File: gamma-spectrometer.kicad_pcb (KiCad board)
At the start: 2 copper layers, 123.5 x 49.5 mm, 79 parts, among them J1 *, J2 *, J3 20449-001E-03, J4 *, J5 20449-001E-03, J6 *, Q1 2N7002, Q2 2N7002, Q3 MMBT5088LT1G, Q4 MMBT5088LT1G, SW1 *, U1 Pico 2, U10 MICROFC-60035-SMT-TR1, U2 OPA357AIDBVR, U3 TLV3201AIDBVR, U4 OPA357AIDBVR, U5 OPA357AIDBVR, U6 LM4040AIM3-3.0+T, U7 LM4040AIM3-3.0+T, U8 MAX5026EUT_T, U9 TPS7B6950DBVR

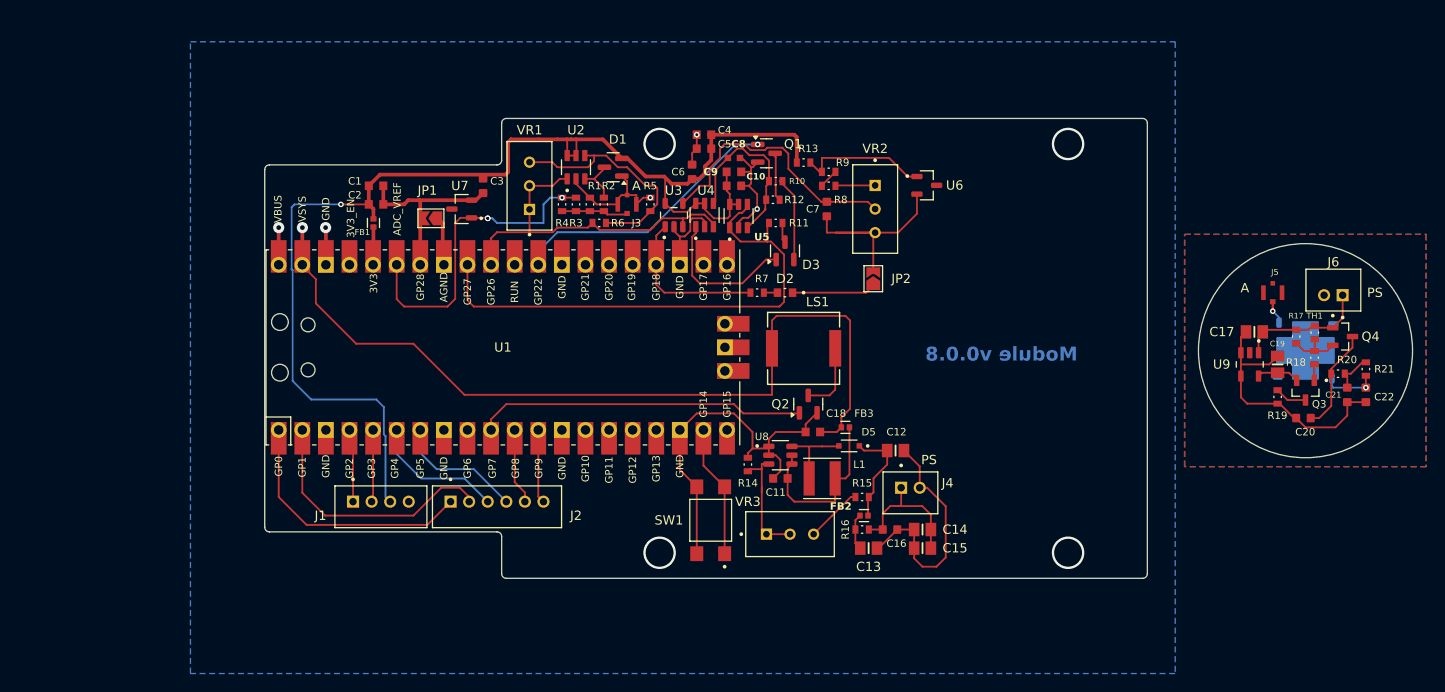
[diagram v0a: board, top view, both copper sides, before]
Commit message: BDG4-01 module boards design
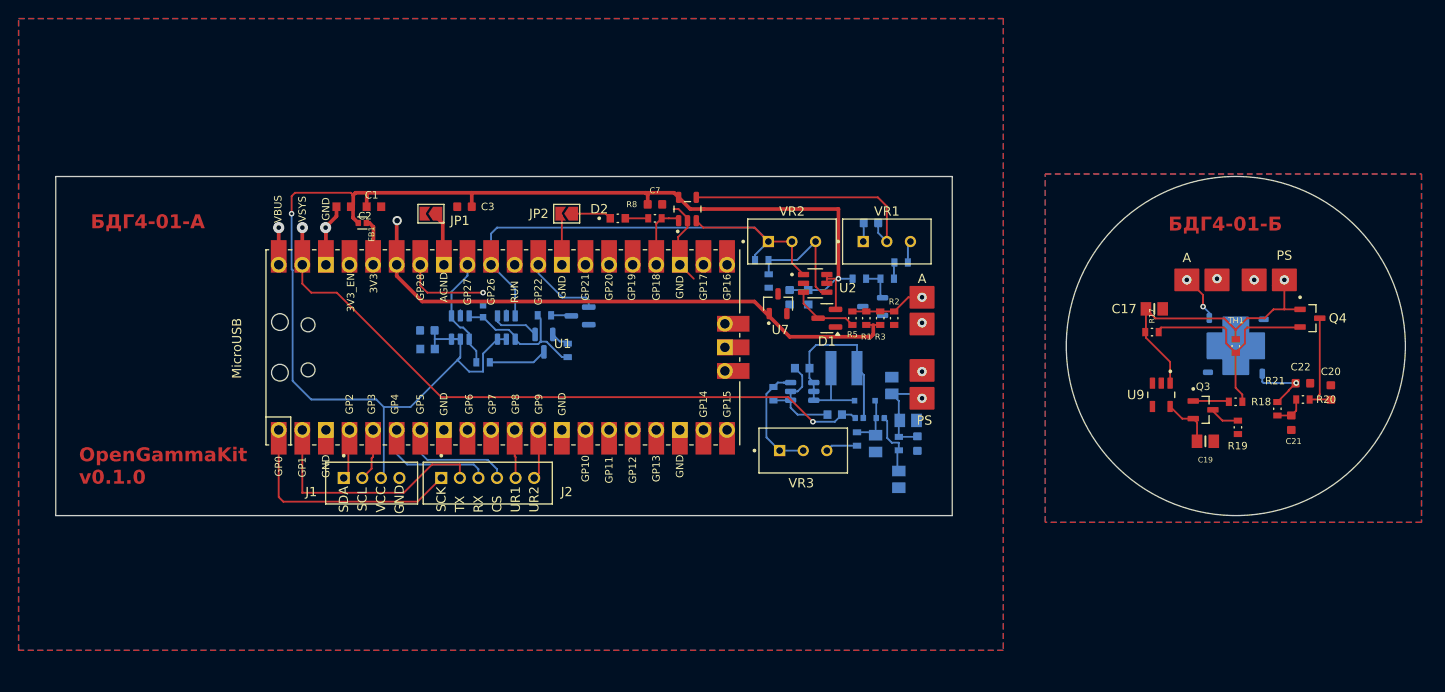
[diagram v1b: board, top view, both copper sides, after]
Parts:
- removed J3, J5: 20449-001E-03, 20449-001E-03:IPEX_20449-001E-03
- removed J4, J6: *, B2B-PH-K-S_LF__SN_:JST_B2B-PH-K-S(LF)(SN)
- removed LS1: AST0760MCTRQ (6kHz), AST0760MCTRQ:AST0760_MAL
- removed Q2: 2N7002, Package_TO_SOT_SMD:SOT-23
- removed SW1: *, SW_TL3305AF160QG:SW_TL3305AF160QG
- C10, C11, C12, C13, C14, C15, C16, C18, C4, C5, C6, C8, C9, D3, D5, FB2, FB3, L1, Q1, R10, R11, R12, R13, R14, R15, R16, R6, R9, U4, U5, U6, U8: moved to B.Cu
- R1: value 1k -> 210k
- R2: value 100R -> 1k
- R4: value 210k -> 1k; moved to B.Cu
- R5: value 1k -> 100R
- R7: value 1k -> 210k; moved to B.Cu
- R8: value 210k -> 1k
- VR1: value 5k -> 50k; footprint 3296W-1-502LF:TRIM_3296W-1-502LF -> 3296W-1-503LF:TRIM_3296W-1-503LF
- VR2: value 50k -> 5k; footprint 3296W-1-503LF:TRIM_3296W-1-503LF -> 3296W-1-502LF:TRIM_3296W-1-502LF
- moved VR1 38.9 mm to (155.0, 72.5), turned to 0 degrees
- moved C9 38.1 mm to (105.5, 84.1), turned to 180 degrees
- moved C10 36.5 mm to (105.5, 82.1), turned to 0 degrees
- moved U7 35.5 mm to (143.2, 79.2), turned to 90 degrees
- moved R3 35.0 mm to (154.2, 80.8), turned to -90 degrees
- moved R11 34.9 mm to (111.5, 85.5)
- moved JP2 33.7 mm to (120.5, 69.5), turned to 180 degrees
- moved R2 33.6 mm to (155.8, 80.8)
- moved U5 32.3 mm to (109.0, 81.8), turned to -90 degrees
- moved R1 32.2 mm to (152.8, 80.8)
- moved C8 31.6 mm to (111.5, 80.0), turned to -90 degrees
- moved R10 28.9 mm to (120.6, 84.2), turned to -90 degrees
- moved U2 28.6 mm to (147.2, 77.0), turned to 0 degrees
- moved D1 28.2 mm to (148.5, 80.8)
- moved D3 27.8 mm to (118.0, 83.4), turned to -90 degrees
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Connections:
- C11 pad 1: Net-(U8-VCC) -> Net-(D5-A)
- C6 pad 1: GND -> Net-(U3-IN-)
- C6 pad 2: VCC -> GND
- C7 pad 1: Net-(U3-IN-) -> GND
- C7 pad 2: GND -> VCC
- FB3 pad 1: Net-(U8-VCC) -> Net-(D5-A)
- L1 pad 2: Net-(U8-VCC) -> Net-(D5-A)
- R1 pad 1: GND -> ANODE_IN
- R1 pad 2: ANODE_IN -> VREF1
- R13 pad 1: VREF1 -> VREF
- R2 pad 1: ANODE_IN -> GND
- R2 pad 2: Net-(D1-COM) -> ANODE_IN
- R3 pad 2: VREF -> VREF1
- R4 pad 1: ANODE_IN -> GND
- R4 pad 2: VREF -> Net-(U2--IN)
- R5 pad 1: GND -> ANODE_IN
- R5 pad 2: Net-(U2--IN) -> Net-(D1-COM)
- R7 pad 1: Net-(D2-PadA) -> Net-(VR1-CW)
- R7 pad 2: INT -> Net-(R7-Pad2)
- R8 pad 1: Net-(VR2-CCW) -> Net-(D2-PadA)
- R8 pad 2: Net-(R8-Pad2) -> INT
- R9 pad 1: VREF1 -> VREF
- R9 pad 2: Net-(R8-Pad2) -> Net-(R7-Pad2)
- U1 pad 10: TCKR -> unconnected-(U1-GPIO7-Pad10)_1
- U1 pad 19: Net-(U1-GPIO14) -> unconnected-(U1-GPIO14-Pad19)_1
- U1 pad 35: VREF -> VREF1
- U1 pad 40: unconnected-(U1-VBUS-Pad40) -> VBUS
- U6 pad 1: VREF1 -> VREF
- U7 pad 1: VREF -> VREF1
- U8 pad 4: Net-(U8-VCC) -> Net-(D5-A)
- U8 pad 5: Net-(U8-VCC) -> Net-(D5-A)
- VR1 pad 1: SIG -> GND
- VR1 pad 2: SIG -> Net-(U3-IN-)
- VR1 pad 3: Net-(U2--IN) -> Net-(VR1-CW)
- VR2 pad 1: Net-(VR2-CCW) -> SIG
- VR2 pad 2: Net-(U3-IN-) -> SIG
- VR2 pad 3: GND -> Net-(U2--IN)
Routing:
- net GND: track 151.7 -> 49.2 mm
- net VREF1: track 14.2 -> 62.6 mm, vias 0 -> 1
- net PEAK: track 56.2 -> 13.6 mm
- net TCKR: track 35.5 -> 0.00 mm
- net VREF: track 34.5 -> 3.69 mm, vias 3 -> 0
- net GND1: track 29.1 -> 0.00 mm, vias 0 -> 2
- net RST: track 29.9 -> 7.38 mm, vias 1 -> 0
- net +5V: track 93.2 -> 72.4 mm, vias 1 -> 2
- net SIG: track 39.7 -> 59.5 mm
- net VCC: track 134.0 -> 153.5 mm, vias 1 -> 2
- net Net-(U8-VCC): track 19.5 -> 0.00 mm
- net Net-(Q4-B): track 5.79 -> 24.9 mm
- net Net-(D5-A): track 9.71 -> 28.3 mm
- net PS_IN: track 14.1 -> 31.9 mm, vias 0 -> 1
- net Net-(U2--IN): track 25.4 -> 13.7 mm
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- added copper zone on F.Cu, net GND
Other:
- board size 123.5 x 49.5 mm -> 145.3 x 36.5 mm
- board text added: "CS"
- board text added: "GND"
- board text added: "MicroUSB"
- board text added: "OpenGammaKit v0.1.0"
- board text added: "RX"
- board text added: "SCK"
- board text added: "SCL"
- board text added: "SDA"
- board text added: "TX"
- board text added: "UR1"
- board text added: "UR2"
- board text added: "VCC"
- board text added: "БДГ4-01-А"
- board text added: "БДГ4-01-Б"
- board text removed: "Module v0.0.8"
- board text removed: "U2"
